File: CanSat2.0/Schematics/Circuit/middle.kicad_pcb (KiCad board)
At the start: 2 copper layers, 64 x 64 mm, 34 parts, among them IC1 ATMEGA2560-A, J1 Conn_02x05_Counter_Clockwise, J2 Conn_02x08_Counter_Clockwise, J3 Conn_01x08, J4 Conn_02x07_Counter_Clockwise, J5 Conn_01x04, Q1 BSS138, Q2 BSS138, Q3 BSS138, Q4 BSS138, U1 SD

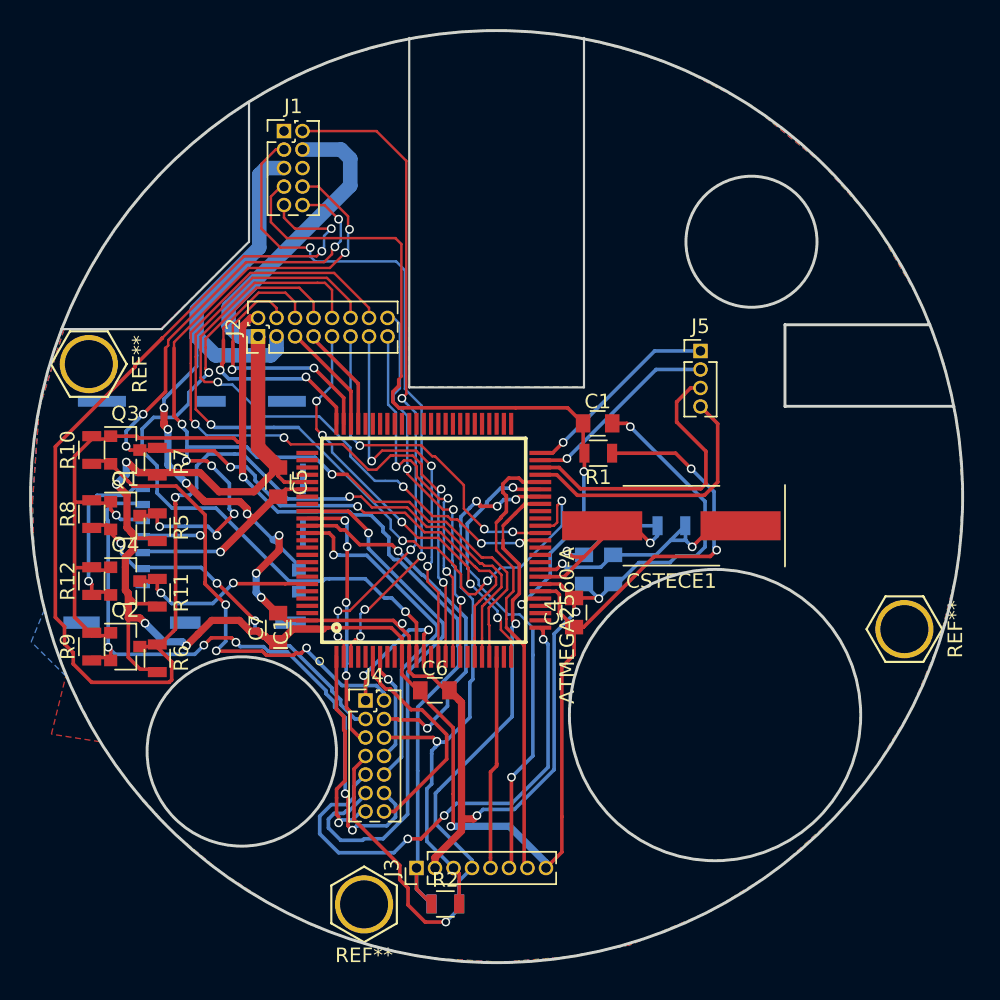
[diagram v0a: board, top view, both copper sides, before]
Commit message: Middle-conectors
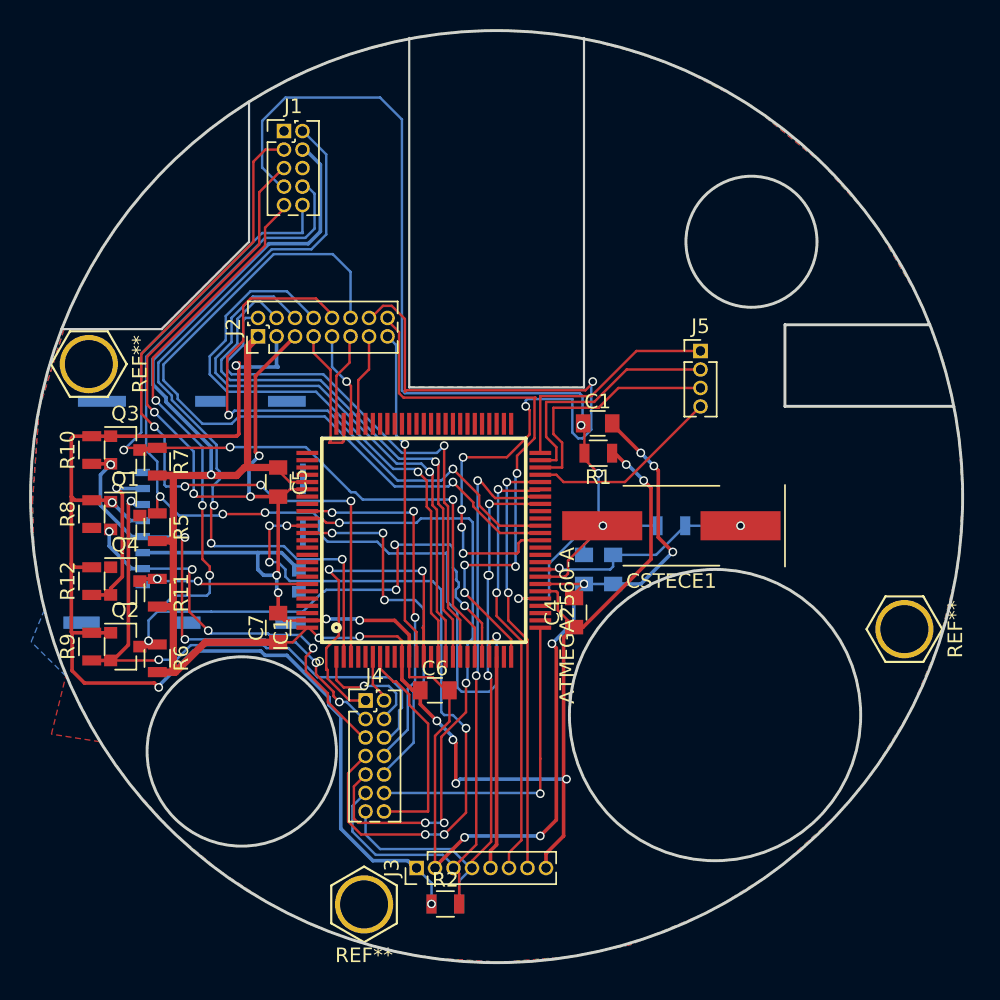
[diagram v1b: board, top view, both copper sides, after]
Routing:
- net /MOSI: track 102.3 -> 73.3 mm, vias 4 -> 7
- net /FC_PWM_6: track 23.6 -> 52.0 mm, vias 3 -> 1
- net /GSM_TX: track 48.2 -> 22.8 mm, vias 2 -> 1
- net /CO2: track 18.5 -> 43.0 mm
- net /O2: track 25.4 -> 48.4 mm, vias 2 -> 6
- net /GSM_RX: track 9.53 -> 26.2 mm
- net /FC_PWM_5: track 57.1 -> 40.9 mm, vias 4 -> 2
- net /FC_PWM_4: track 27.0 -> 42.3 mm, vias 3 -> 1
- net /GSM_SLP: track 20.5 -> 6.40 mm, vias 2 -> 0
- net /RST: track 53.0 -> 66.9 mm, vias 2 -> 3
- net /FC_PWM_3: track 53.8 -> 40.5 mm, vias 4 -> 1
- net /FC_PWM_2: track 25.7 -> 38.9 mm, vias 3 -> 1
- net /O3: track 37.8 -> 25.1 mm, vias 1 -> 3
- net /SERVO: track 34.5 -> 22.2 mm, vias 3 -> 1
- net /RFM_INT: track 15.5 -> 3.32 mm
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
